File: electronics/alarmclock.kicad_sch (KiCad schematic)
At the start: 41 parts, among them J1 Conn_01x02, J2 SWD, J3 SocketTop, J4 SocketBottem, J5 Conn_01x02, J6 Conn_01x05, J7 Conn_01x05, Q1 Backpower, SW1 RotaryEncoder_Switch, SW2 Reset, U1 STM32L031F6P6, U2 74HCT595, U3 74HCT595, U4 AP2111H-3.3, Y1 24MHz

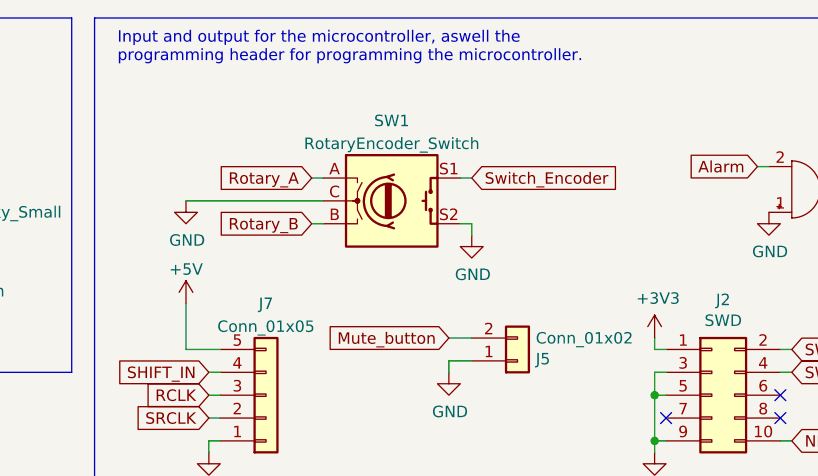
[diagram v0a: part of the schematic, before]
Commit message: finilised for review
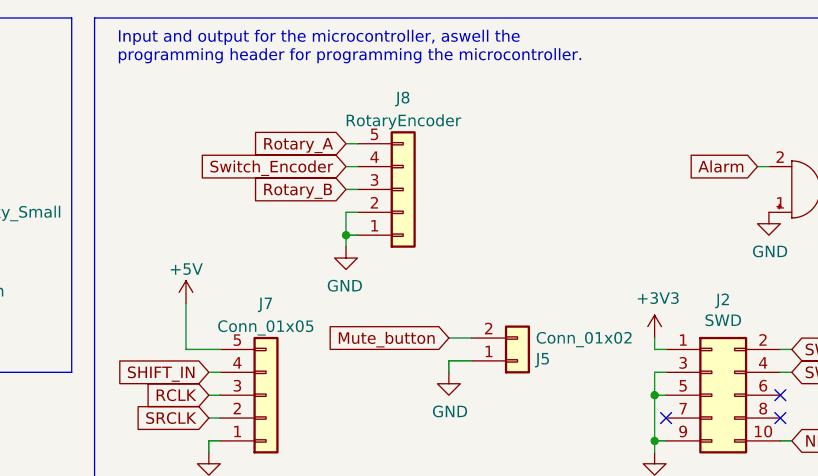
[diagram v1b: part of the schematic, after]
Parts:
- removed SW1: RotaryEncoder_Switch, Rotary_Encoder:RotaryEncoder_Bourns_Horizontal_PEC09-2xxxF-Nxxxx, symbol Device:RotaryEncoder_Switch
- added J8: RotaryEncoder, Connector_PinHeader_2.54mm:PinHeader_1x05_P2.54mm_Vertical, symbol Connector_Generic:Conn_01x05
- BT1: footprint (none) -> Battery:BatteryHolder_ComfortableElectronic_CH273-2450_1x2450
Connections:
- net GND: now also J8.1 (Pin_1), J8.2 (Pin_2)
- net Rotary_A: now also J8.5 (Pin_5)
- net Rotary_B: now also J8.3 (Pin_3)
- net Switch_Encoder: now also J8.4 (Pin_4)
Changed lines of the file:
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@@
   (junction (at 81.28 30.48) (diameter 0) (color 0 0 0 0)
+  )
+  (junction (at 148.59 38.1) (diameter 0) (color 0 0 0 0)
   )
   (junction (at 52.07 68.58) (diameter 0) (color 0 0 0 0)
@@
     (stroke (width 0) (type default))
   )
-  (wire (pts (xy 161.29 36.83) (xy 162.56 36.83))
+  (wire (pts (xy 149.86 38.1) (xy 148.59 38.1))
     (stroke (width 0) (type default))
   )
@@
     (stroke (width 0) (type default))
   )
-  (wire (pts (xy 162.56 31.75) (xy 161.29 31.75))
+  (wire (pts (xy 148.59 35.56) (xy 149.86 35.56))
     (stroke (width 0) (type default))
   )
@@
     (stroke (width 0) (type default))
   )
-  (wire (pts (xy 130.81 34.29) (xy 146.05 34.29))
-    (stroke (width 0) (type default))
-  )
   (wire (pts (xy 189.23 124.46) (xy 187.96 124.46))
     (stroke (width 0) (type default))
@@
     (stroke (width 0) (type default))
   )
-  (wire (pts (xy 144.78 31.75) (xy 146.05 31.75))
+  (wire (pts (xy 148.59 27.94) (xy 149.86 27.94))
     (stroke (width 0) (type default))
   )
@@
     (stroke (width 0) (type default))
   )
-  (wire (pts (xy 162.56 36.83) (xy 162.56 38.1))
+  (wire (pts (xy 148.59 38.1) (xy 148.59 39.37))
     (stroke (width 0) (type default))
   )
@@
     (stroke (width 0) (type default))
   )
+  (wire (pts (xy 148.59 30.48) (xy 149.86 30.48))
+    (stroke (width 0) (type default))
+  )
   (wire (pts (xy 120.65 101.6) (xy 130.81 101.6))
     (stroke (width 0) (type default))
@@
     (stroke (width 0) (type default))
   )
-  (wire (pts (xy 144.78 36.83) (xy 146.05 36.83))
+  (wire (pts (xy 148.59 33.02) (xy 149.86 33.02))
     (stroke (width 0) (type default))
   )
@@
   )
   (wire (pts (xy 219.71 114.3) (xy 220.98 114.3))
+    (stroke (width 0) (type default))
+  )
+  (wire (pts (xy 148.59 35.56) (xy 148.59 38.1))
     (stroke (width 0) (type default))
   )
@@
     )
   )
-  (global_label "Rotary_B" (shape input) (at 144.78 36.83 180)
+  (global_label "Rotary_B" (shape input) (at 148.59 33.02 180)
     (effects (font (size 1.27 1.27)) (justify right))
-    (property "Intersheetrefs" "${INTERSHEET_REFS}" (at 144.78 36.83 0)
-      (effects (font (size 1.27 1.27)) hide)
-    )
-  )
-  (global_label "Switch_Encoder" (shape input) (at 162.56 31.75 0)
-    (effects (font (size 1.27 1.27)) (justify left))
-    (property "Intersheetrefs" "${INTERSHEET_REFS}" (at 162.56 31.75 0)
+    (property "Intersheetrefs" "${INTERSHEET_REFS}" (at 148.59 33.02 0)
+      (effects (font (size 1.27 1.27)) hide)
+    )
+  )
+  (global_label "Switch_Encoder" (shape input) (at 148.59 30.48 180)
+    (effects (font (size 1.27 1.27)) (justify right))
+    (property "Intersheetrefs" "${INTERSHEET_REFS}" (at 148.59 30.48 0)
       (effects (font (size 1.27 1.27)) hide)
     )
@@
     )
   )
-  (global_label "Rotary_A" (shape input) (at 144.78 31.75 180)
+  (global_label "Rotary_A" (shape input) (at 148.59 27.94 180)
     (effects (font (size 1.27 1.27)) (justify right))
-    (property "Intersheetrefs" "${INTERSHEET_REFS}" (at 144.78 31.75 0)
+    (property "Intersheetrefs" "${INTERSHEET_REFS}" (at 148.59 27.94 0)
       (effects (font (size 1.27 1.27)) hide)
     )
@@
     )
   )
-  (symbol (lib_id "power:GND") (at 162.56 38.1 0) (unit 1)
-    (in_bom yes) (on_board yes) (dnp no)
-    (property "Reference" "#PWR07" (at 162.56 44.45 0)
-      (effects (font (size 1.27 1.27)) hide)
-    )
-    (property "Value" "GND" (at 162.687 42.4942 0)
-      (effects (font (size 1.27 1.27)))
-    )
-    (property "Footprint" "" (at 162.56 38.1 0)
-      (effects (font (size 1.27 1.27)) hide)
-    )
-    (property "Datasheet" "" (at 162.56 38.1 0)
+  (symbol (lib_id "power:GND") (at 148.59 39.37 0) (mirror y) (unit 1)
+    (in_bom yes) (on_board yes) (dnp no)
+    (property "Reference" "#PWR07" (at 148.59 45.72 0)
+      (effects (font (size 1.27 1.27)) hide)
+    )
+    (property "Value" "GND" (at 148.463 43.7642 0)
+      (effects (font (size 1.27 1.27)))
+    )
+    (property "Footprint" "" (at 148.59 39.37 0)
+      (effects (font (size 1.27 1.27)) hide)
+    )
+    (property "Datasheet" "" (at 148.59 39.37 0)
       (effects (font (size 1.27 1.27)) hide)
     )
@@
       (effects (font (size 1.27 1.27)) (justify left))
     )
-    (property "Footprint" "" (at 99.06 42.926 90)
+    (property "Footprint" "Battery:BatteryHolder_ComfortableElectronic_CH273-2450_1x2450" (at 99.06 42.926 90)
       (effects (font (size 1.27 1.27)) hide)
     )
@@
         (path "/fcd099cf-d7c6-418d-b6d0-a7fbd5aabc64"
           (reference "R1") (unit 1)
-        )
-      )
-    )
-  )
-  (symbol (lib_id "power:GND") (at 130.81 34.29 0) (unit 1)
-    (in_bom yes) (on_board yes) (dnp no)
-    (property "Reference" "#PWR0106" (at 130.81 40.64 0)
-      (effects (font (size 1.27 1.27)) hide)
-    )
-    (property "Value" "GND" (at 130.937 38.6842 0)
-      (effects (font (size 1.27 1.27)))
-    )
-    (property "Footprint" "" (at 130.81 34.29 0)
-      (effects (font (size 1.27 1.27)) hide)
-    )
-    (property "Datasheet" "" (at 130.81 34.29 0)
-      (effects (font (size 1.27 1.27)) hide)
-    )
-    (pin "1")
-    (instances
-      (project "alarmclock"
-        (path "/fcd099cf-d7c6-418d-b6d0-a7fbd5aabc64"
-          (reference "#PWR0106") (unit 1)
         )
       )
@@
     )
   )
-  (symbol (lib_id "Device:RotaryEncoder_Switch") (at 153.67 34.29 0) (unit 1)
-    (in_bom yes) (on_board yes) (dnp no) (fields_autoplaced)
-    (property "Reference" "SW1" (at 153.67 25.4 0)
-      (effects (font (size 1.27 1.27)))
-    )
-    (property "Value" "RotaryEncoder_Switch" (at 153.67 27.94 0)
-      (effects (font (size 1.27 1.27)))
-    )
-    (property "Footprint" "Rotary_Encoder:RotaryEncoder_Bourns_Horizontal_PEC09-2xxxF-Nxxxx" (at 149.86 30.226 0)
-      (effects (font (size 1.27 1.27)) hide)
-    )
-    (property "Datasheet" "~" (at 153.67 27.686 0)
-      (effects (font (size 1.27 1.27)) hide)
-    )
-    (pin "A")
-    (pin "B")
-    (pin "C")
-    (pin "S1")
-    (pin "S2")
-    (instances
-      (project "alarmclock"
-        (path "/fcd099cf-d7c6-418d-b6d0-a7fbd5aabc64"
-          (reference "SW1") (unit 1)
-        )
-      )
-    )
-  )
   (symbol (lib_id "Device:R_Small") (at 191.77 114.3 270) (mirror x) (unit 1)
     (in_bom yes) (on_board yes) (dnp no)
@@
         )
       )
+    )
+  )
+  (symbol (lib_id "Connector_Generic:Conn_01x05") (at 154.94 33.02 0) (mirror x) (unit 1)
+    (in_bom yes) (on_board yes) (dnp no)
+    (property "Reference" "J8" (at 154.94 22.86 0)
+      (effects (font (size 1.27 1.27)))
+    )
+    (property "Value" "RotaryEncoder" (at 154.94 25.4 0)
+      (effects (font (size 1.27 1.27)))
+    )
+    (property "Footprint" "Connector_PinHeader_2.54mm:PinHeader_1x05_P2.54mm_Vertical" (at 154.94 33.02 0)
+      (effects (font (size 1.27 1.27)) hide)
+    )
+    (property "Datasheet" "~" (at 154.94 33.02 0)
+      (effects (font (size 1.27 1.27)) hide)
+    )
+    (pin "1")
+    (pin "2")
+    (pin "3")
+    (pin "4")
+    (pin "5")
+    (instances
+      (project "alarmclock"
+        (path "/fcd099cf-d7c6-418d-b6d0-a7fbd5aabc64"
+          (reference "J8") (unit 1)
+        )
+      )
